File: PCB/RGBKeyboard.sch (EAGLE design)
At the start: 1 part, among them U1 MSP430F5529_PN_80

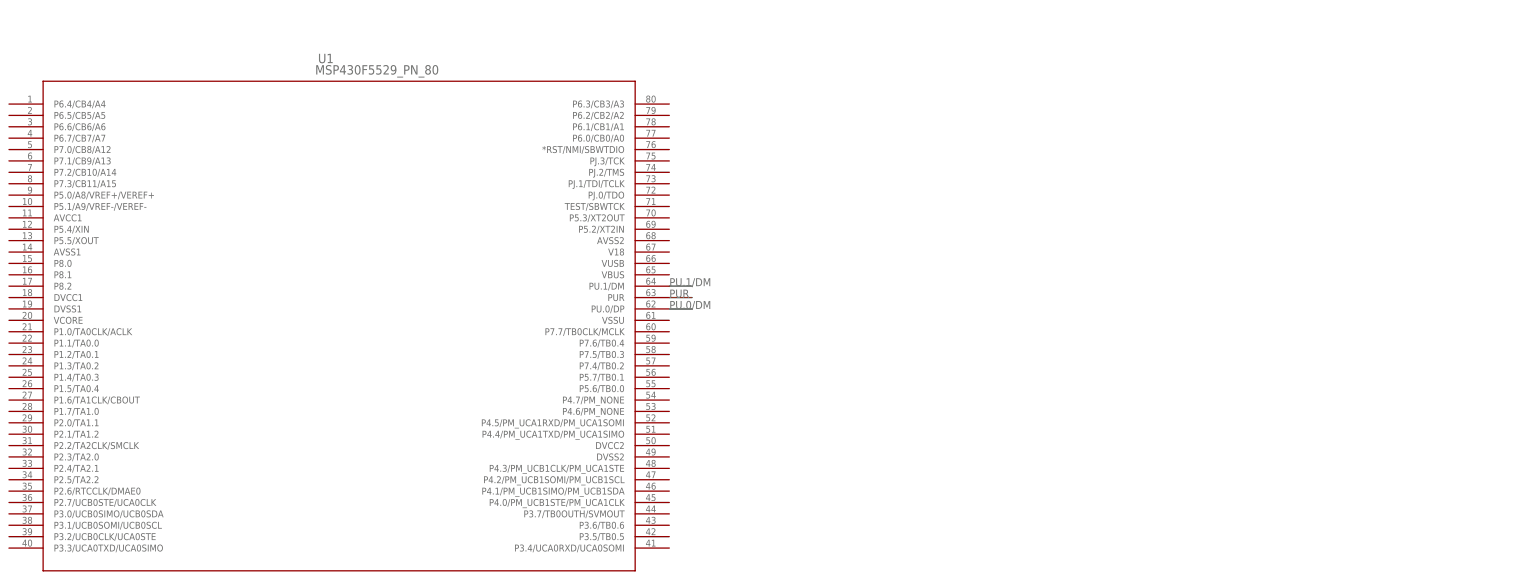
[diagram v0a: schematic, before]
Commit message: USB lib and schematic
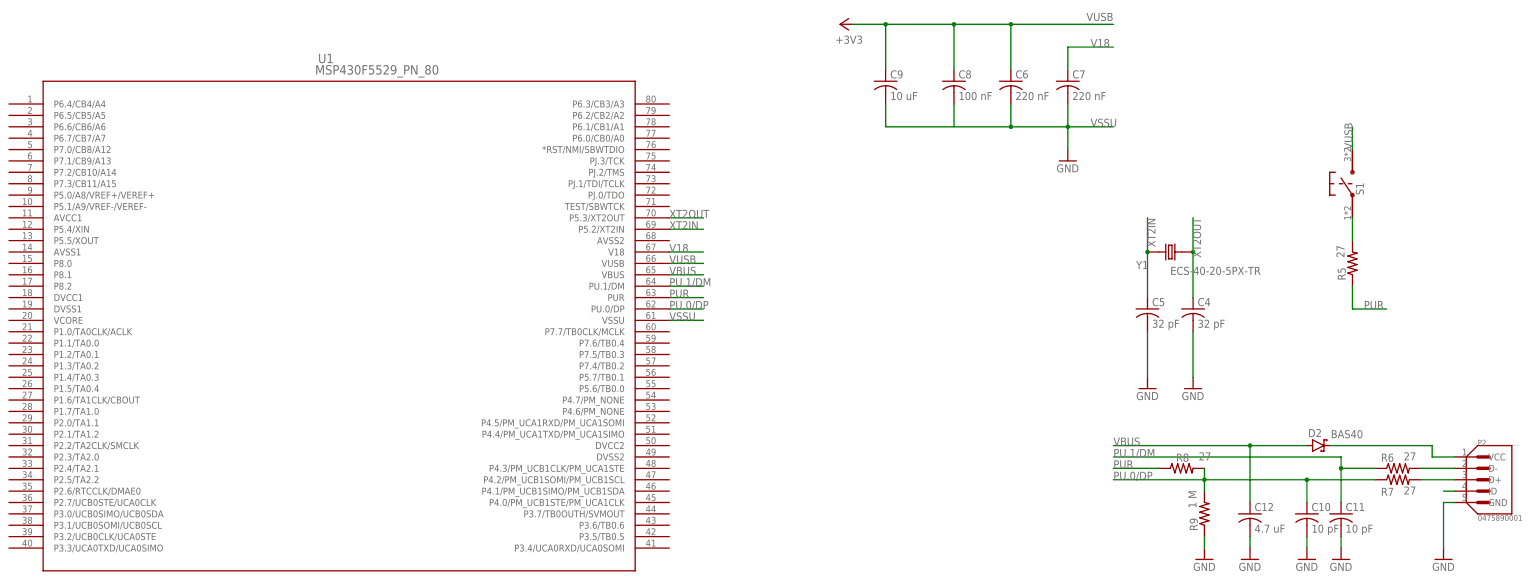
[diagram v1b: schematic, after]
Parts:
- added C10, C11: 10 pF, rcl:C-USC0603K
- added C12: 4.7 uF, rcl:C-USC0603K
- added C4, C5: 32 pF, rcl:C-USC0603K
- added C6, C7: 220 nF, rcl:C-USC0603K
- added C8: 100 nF, rcl:C-USC0603K
- added C9: 10 uF, rcl:C-USC0603K
- added D2: BAS40, diode:BAS40
- added P2: 0475890001, MICRO_USB_B:0475890001
- added R5, R6, R7, R8: 27, rcl:R-US_R0603
- added R9: 1 M, rcl:R-US_R0603
- added S1: PTS645SM43SMTR, PTS645SM43SMTR:PTS645SM43SMTR
- added Y1: ECS-40-20-5PX-TR, ECS-40-20-5PX-TR:ECS-40-20-5PX-TR
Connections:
- removed net PU.0/DM: U1.PU.0/DP
- new net GND: C10.2, C11.2, C12.2, C4.2, C5.2, P2.GND, R9.1
- new net N$10: D2.C, P2.VCC
- new net N$4: R5.2, S1.P$1
- new net N$5: C8.2
- new net N$7: P2.ID
- new net N$8: P2.D-, R6.2
- new net N$9: P2.D+, R7.2
- new net PU.0/DP: C10.1, R7.1, R8.2, R9.2, U1.PU.0/DP
- new net V18: C7.1, U1.V18
- new net VBUS: C12.1, D2.A, U1.VBUS
- new net VSSU: C6.2, C7.2, C9.2, U1.VSSU
- new net VUSB: C6.1, C8.1, C9.1, S1.P$2, U1.VUSB
- new net XT2IN: C5.1, U1.P5.2/XT2IN, Y1.1
- new net XT2OUT: C4.1, U1.P5.3/XT2OUT, Y1.2
- net PU.1/DM: now also C11.1, R6.1
- net PUR: now also R5.1, R8.1
